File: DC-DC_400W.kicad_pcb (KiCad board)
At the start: 2 copper layers, 82 x 63 mm, 15 parts, among them J1 Conn_01x24, J11 Conn_01x06, J12 Conn_01x06, J2 Conn_01x03, J4 Conn_01x01, J5 Conn_01x01, J6 Conn_01x02, J7 Conn_01x01, J8 Conn_01x01, J9 Conn_01x01

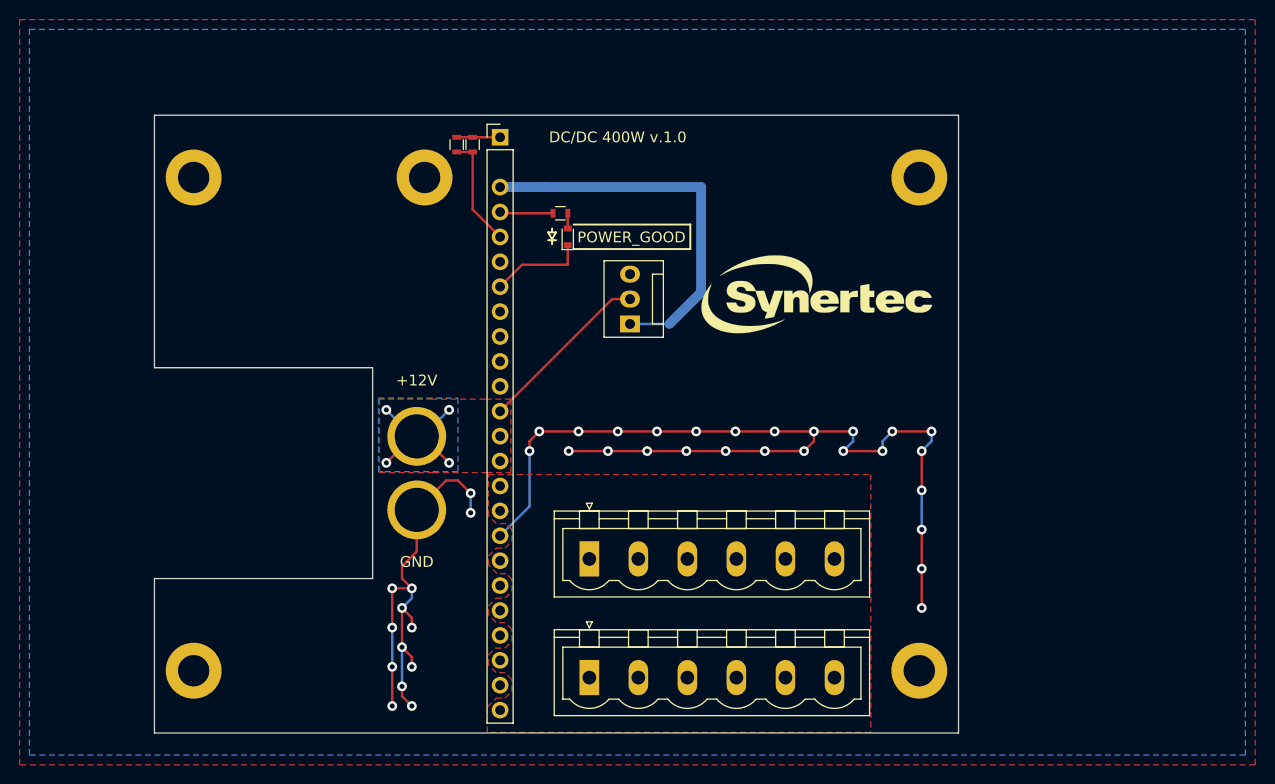
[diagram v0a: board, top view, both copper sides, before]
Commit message: 0.35mm/0.35mm
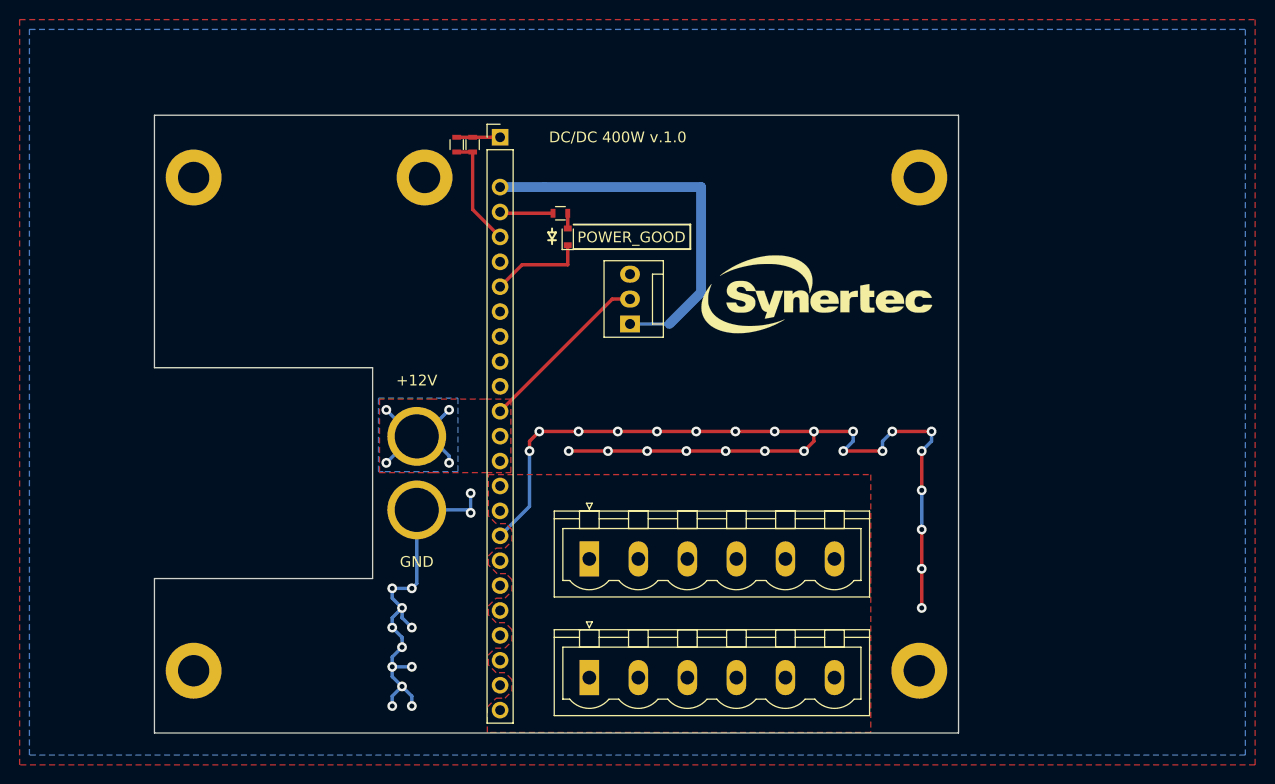
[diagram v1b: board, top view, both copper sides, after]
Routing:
- net GND: track 201.6 -> 190.7 mm
- net +12V: track 34.6 -> 35.3 mm
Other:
- net class Default: clearance 0.25 -> 0.35; trace_width 0.25 -> 0.35
- rule trace_clearance: 0.25 -> 0.35
- rule trace_min: 0.25 -> 0.35
